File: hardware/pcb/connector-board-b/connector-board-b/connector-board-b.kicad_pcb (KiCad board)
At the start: 2 copper layers, 21.3 x 50.5 mm, 4 parts, among them J1 DE9_Pins, J3 Conn_01x02, J4 Conn_01x02, J5 8-215570-0

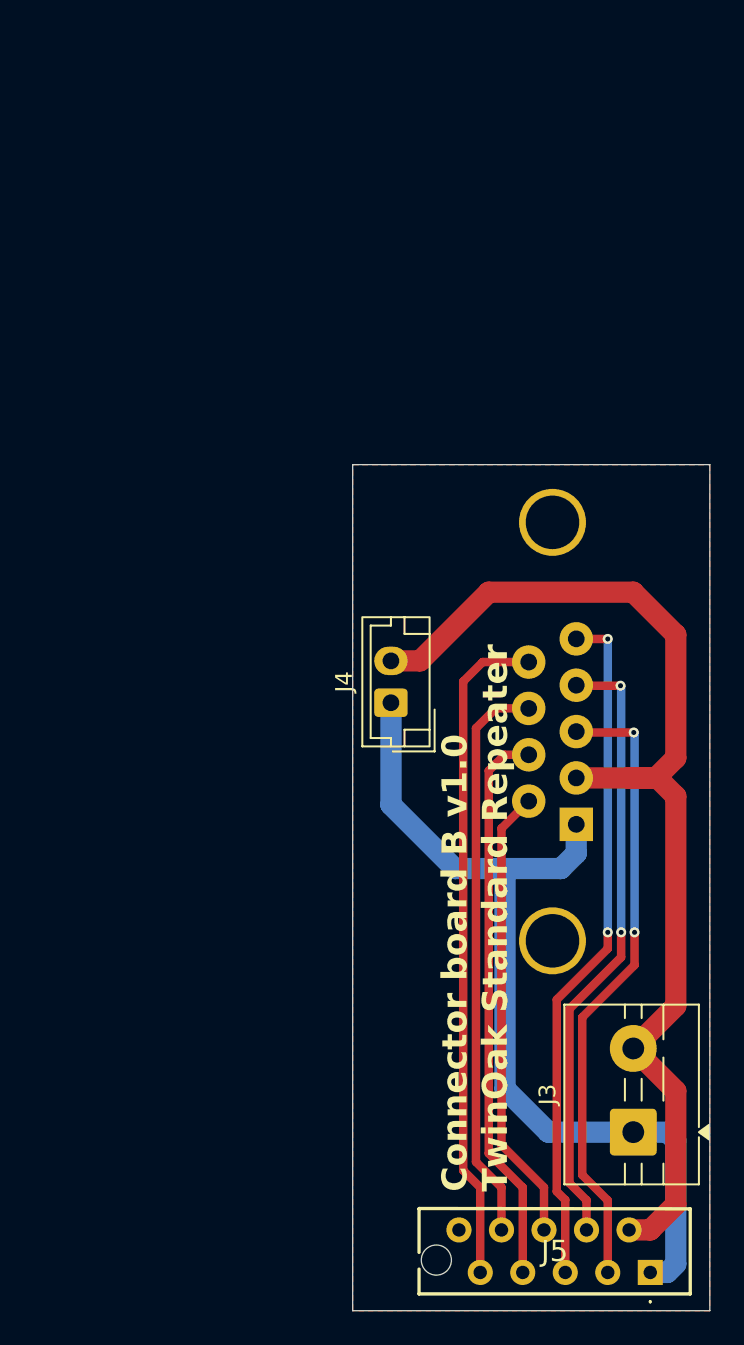
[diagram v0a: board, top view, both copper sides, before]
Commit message: Updated Connectorboard B to rev. 1.1
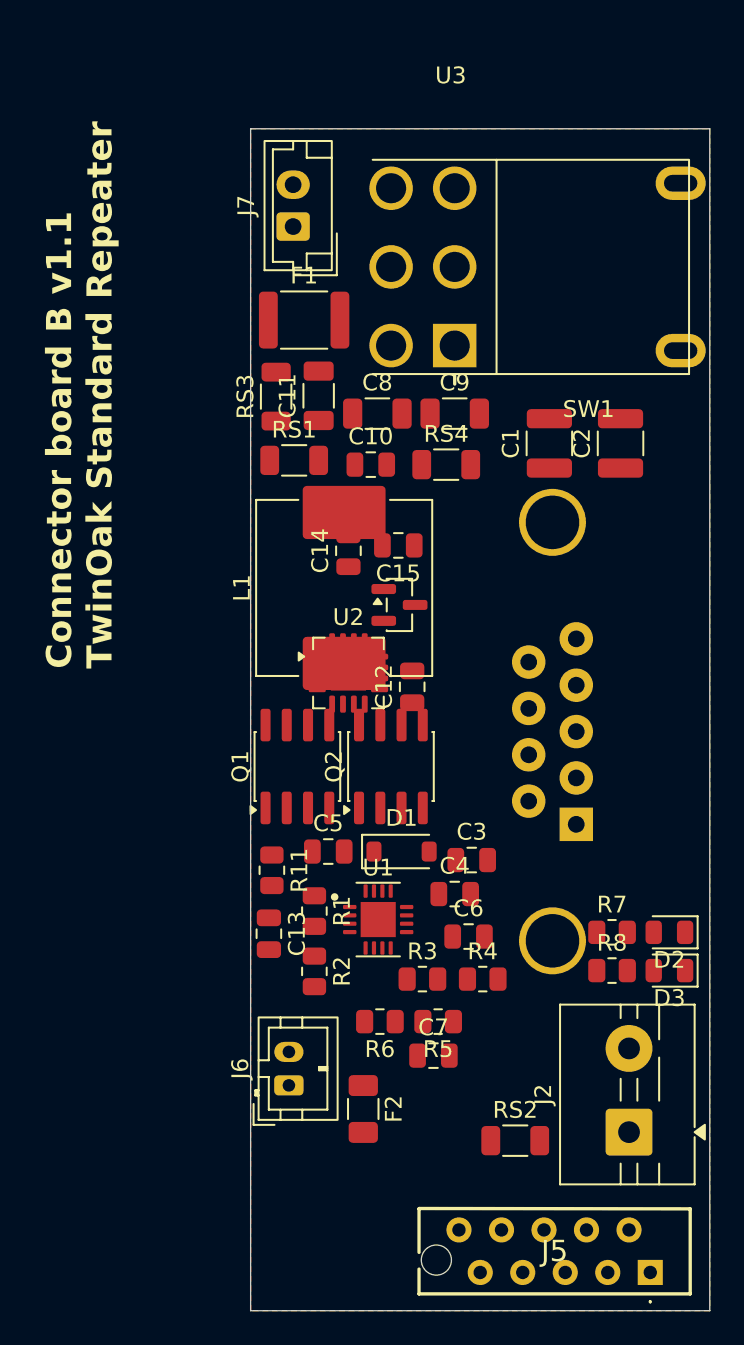
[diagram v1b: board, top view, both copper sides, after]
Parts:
- removed J3: Conn_01x02, TerminalBlock:TerminalBlock_MaiXu_MX126-5.0-02P_1x02_P5.00mm
- removed J4: Conn_01x02, Connector_JST:JST_EH_B2B-EH-A_1x02_P2.50mm_Vertical
- added C1: 10u 50V, Capacitor_SMD:C_1210_3225Metric, F.Cu at (159.1, 49.8)
- added C10: 100n, Capacitor_SMD:C_0805_2012Metric, F.Cu at (148.4, 51.1)
- added C11: 10u, Capacitor_SMD:C_1206_3216Metric, F.Cu at (145.3, 46.9)
- added C12: 100n, Capacitor_SMD:C_0805_2012Metric, F.Cu at (150.9, 64.3)
- added C13: 1n DNP, Capacitor_SMD:C_0805_2012Metric, F.Cu at (142.3, 79.1)
- added C14: 1u, Capacitor_SMD:C_0805_2012Metric, F.Cu at (147.1, 56.2)
- added C15: 1u, Capacitor_SMD:C_0805_2012Metric, F.Cu at (150.0, 55.9)
- added C2: 10u 50V, Capacitor_SMD:C_1210_3225Metric, F.Cu at (163.3, 49.8)
- added C3: 100n, Capacitor_SMD:C_0805_2012Metric, F.Cu at (154.4, 74.7)
- added C4: 1u, Capacitor_SMD:C_0805_2012Metric, F.Cu at (153.4, 76.7)
- added C5: 100n, Capacitor_SMD:C_0805_2012Metric, F.Cu at (145.9, 74.2)
- added C6: 1u, Capacitor_SMD:C_0805_2012Metric, F.Cu at (154.2, 79.2)
- added C7: 1u, Capacitor_SMD:C_0805_2012Metric, F.Cu at (152.1, 86.4)
- added C8: 10u, Capacitor_SMD:C_1206_3216Metric, F.Cu at (148.8, 48.0)
- added C9: 10u, Capacitor_SMD:C_1206_3216Metric, F.Cu at (153.4, 48.0)
- added D1: BAT42W, Diode_SMD:D_SOD-123, F.Cu at (150.2, 74.2)
- added D2: CHG (RED), LED_SMD:LED_0805_2012Metric, F.Cu at (166.2, 79.0)
- added D3: DONE (GRN), LED_SMD:LED_0805_2012Metric, F.Cu at (166.2, 81.3)
- added F1: PTC 3A (SMD1812P300TF/16), Fuse:Fuse_1812_4532Metric, F.Cu at (144.4, 42.4)
- added F2: PTC 0.35A (SMD1206P035TF/30), Fuse:Fuse_1206_3216Metric, F.Cu at (148.0, 89.5)
- added J2: PANEL_18V, TerminalBlock:TerminalBlock_MaiXu_MX126-5.0-02P_1x02_P5.00mm, F.Cu at (163.8, 90.9)
- added J6: NTC_103AT, Connector_JST:JST_PH_B2B-PH-K_1x02_P2.00mm_Vertical, F.Cu at (143.5, 88.1)
- added J7: BATTERY, Connector_JST:JST_EH_B2B-EH-A_1x02_P2.50mm_Vertical, F.Cu at (143.8, 36.8)
- added L1: 10u, Inductor_SMD:L_Vishay_IHLP-4040, F.Cu at (146.8, 58.4)
- added Q1: Si4840BDY, Package_SO:SOIC-8_3.9x4.9mm_P1.27mm, F.Cu at (144.0, 69.1)
- added Q2: Si4840BDY, Package_SO:SOIC-8_3.9x4.9mm_P1.27mm, F.Cu at (149.6, 69.1)
- added R1: 499k 1%, Resistor_SMD:R_0805_2012Metric, F.Cu at (145.0, 77.7)
- added R11: 2R2 DNP, Resistor_SMD:R_0805_2012Metric, F.Cu at (142.5, 75.3)
- added R2: 36k 1%, Resistor_SMD:R_0805_2012Metric, F.Cu at (145.0, 81.3)
- added R3: 499k 1%, Resistor_SMD:R_0805_2012Metric, F.Cu at (151.5, 81.8)
- added R4: 499k 1%, Resistor_SMD:R_0805_2012Metric, F.Cu at (155.1, 81.8)
- added R5: 5k23 1%, Resistor_SMD:R_0805_2012Metric, F.Cu at (152.4, 84.3)
- added R6: 30k1 1%, Resistor_SMD:R_0805_2012Metric, F.Cu at (148.9, 84.3)
- added R7: 2k, Resistor_SMD:R_0805_2012Metric, F.Cu at (162.8, 79.0)
- added R8: 2k, Resistor_SMD:R_0805_2012Metric, F.Cu at (162.8, 81.3)
- added RS1: 0R02 1%, Resistor_SMD:R_1206_3216Metric, F.Cu at (143.8, 50.8)
- added RS2: 0R10 1%, Resistor_SMD:R_1206_3216Metric, F.Cu at (157.0, 91.4)
- added RS3: 0R02 1%, Resistor_SMD:R_1206_3216Metric, F.Cu at (142.7, 47.0)
- added RS4: 0R05 1%, Resistor_SMD:R_1206_3216Metric, F.Cu at (152.9, 51.1)
- added SW1: PWR_KILL, connector-board-b:SW_Toggle_CAX_MTS202C3D1_RightAngle, F.Cu at (153.4, 39.2)
- added U1: BQ24650RVA, solar_charger:Texas_RVA0016A_VQFN-16-1EP_3.5x3.5mm_P0.5mm_EP2.1x2.1mm, F.Cu at (148.8, 78.2)
- added U2: INA3221, Package_DFN_QFN:Texas_RGV0016A_VQFN-16-1EP_4x4mm_P0.65mm_EP2.1x2.1mm, F.Cu at (147.1, 63.5)
- added U3: MCP1700-3.3, Package_TO_SOT_SMD:SOT-23, F.Cu at (150.1, 59.4)
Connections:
- net Net-(J1-Pad3) renamed LORA_nRESET
- net Net-(J1-Pad4) renamed LORA_SWDCLK
- net Net-(J1-Pad5) renamed LORA_SWDIO
- net Net-(J1-Pad6) renamed LORA_PWR_KILL
- net Net-(J1-Pad8) renamed WALTER_TX
- net Net-(J1-Pad9) renamed WALTER_RX
- J1 pad 2: VCC -> VBAT_OUT
- J1 pad 7: Net-(J1-Pad7) -> unconnected-(J1-Pad7)
- J5 pad 10: unconnected-(J5-Pad10) -> I2C_SCL
- J5 pad 2: VCC -> VBAT_RAW
- J5 pad 7: Net-(J1-Pad7) -> I2C_SDA
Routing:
- net VCC: track 66.8 -> 0.00 mm
- net GND: track 54.6 -> 0.00 mm
- net LORA_SWDIO: track 41.2 -> 0.00 mm, vias 2 -> 0
- net WALTER_RX: track 40.1 -> 0.00 mm
- net LORA_nRESET: track 37.7 -> 0.00 mm, vias 2 -> 0
- net LORA_SWDCLK: track 36.9 -> 0.00 mm, vias 2 -> 0
- net WALTER_TX: track 34.2 -> 0.00 mm
- net Net-(J1-Pad7): track 33.6 -> 0.00 mm
- net LORA_PWR_KILL: track 27.3 -> 0.00 mm
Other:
- board size 21.3 x 50.5 mm -> 27.4 x 70.6 mm
- board text added: "Connector board B v1.1 TwinOak Standard Repeater"
- board text removed: "Connector board B v1.0 TwinOak Standard Repeater"
